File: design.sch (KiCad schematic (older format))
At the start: 20 parts, among them J1 USB_C_Receptacle, J2 Conn_01x05, Q1 2N7002K, Q2 2N7002K, Q3 2N7002K, U1 ATtiny814-SS

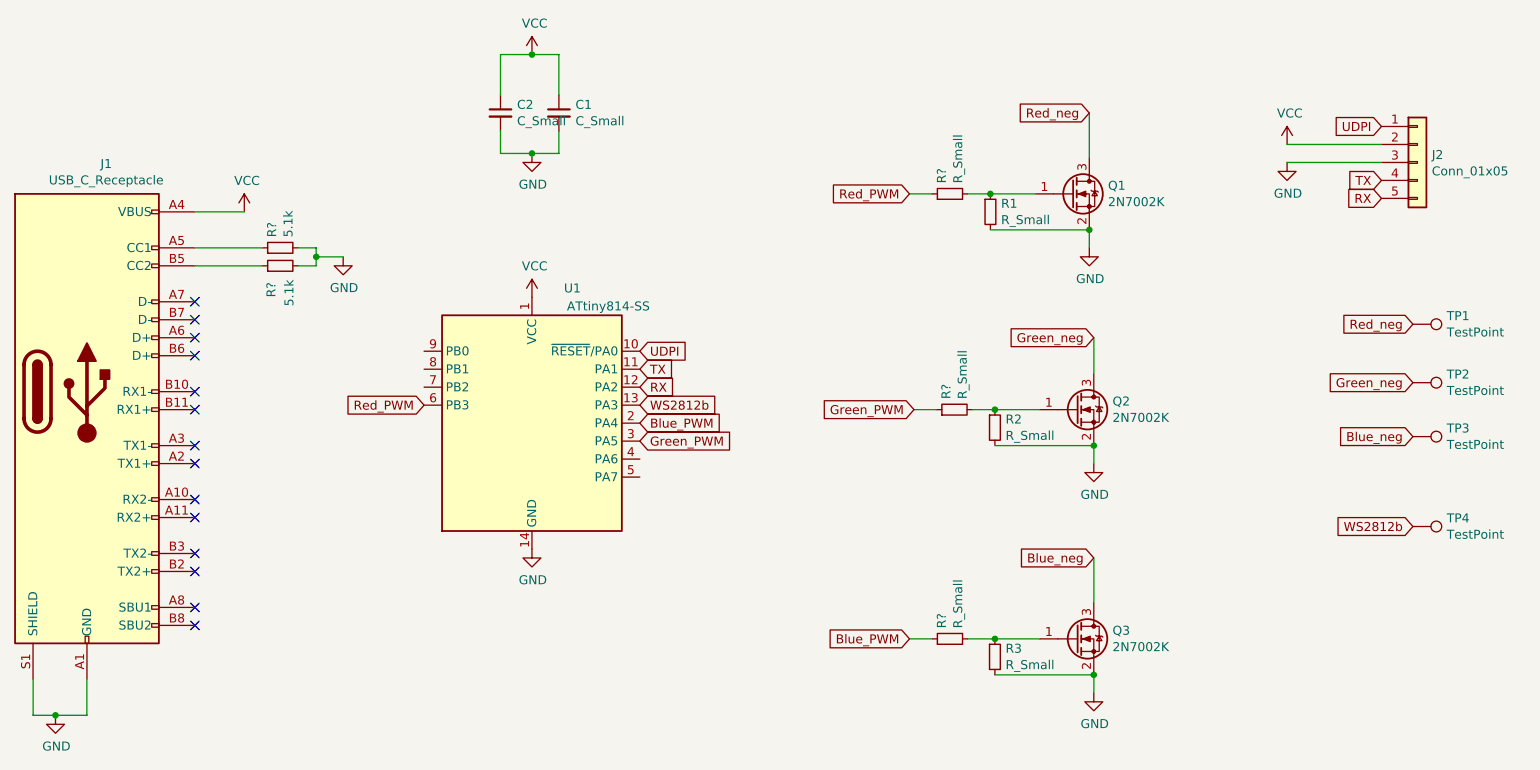
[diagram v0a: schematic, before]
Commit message: simple usb c footprint
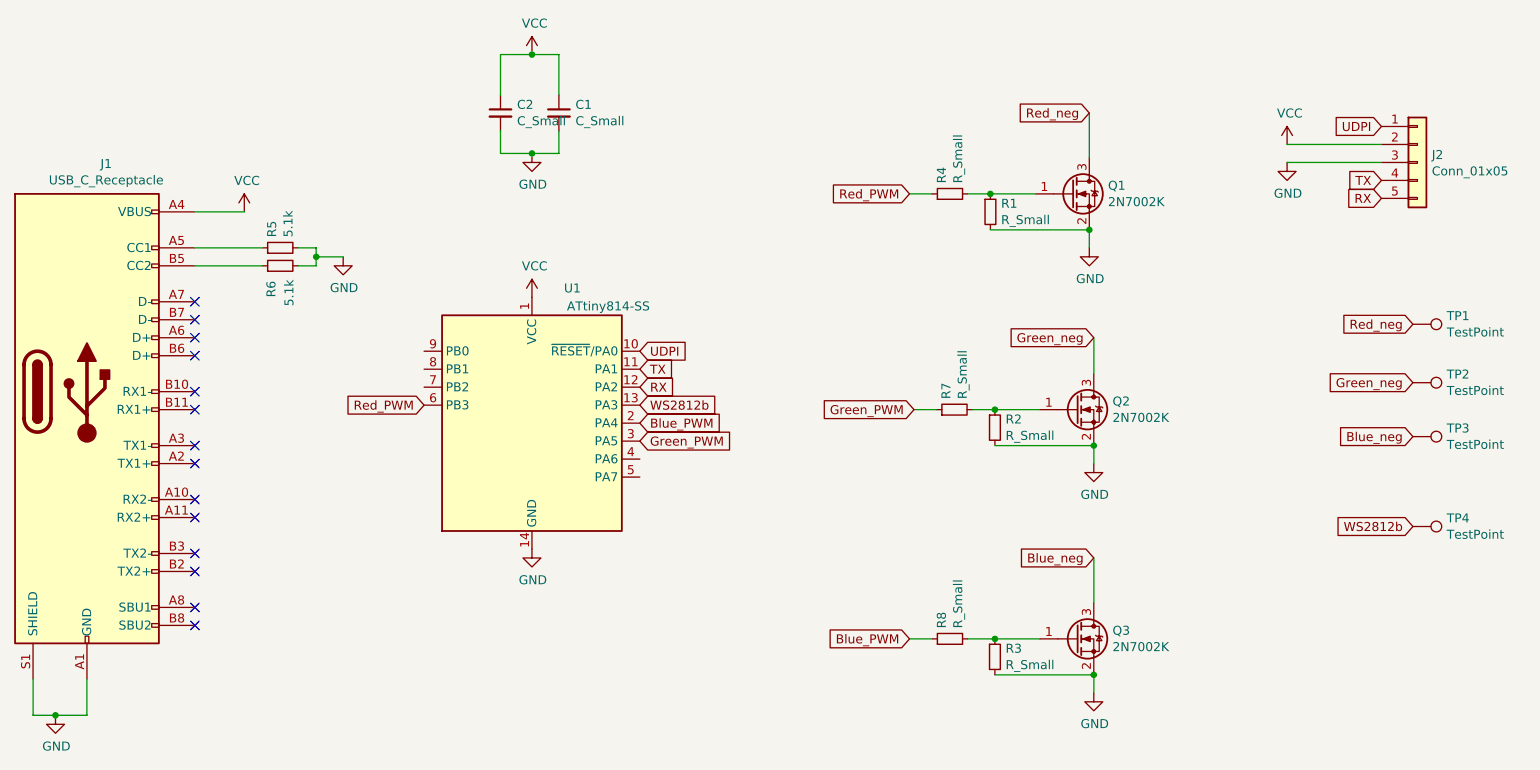
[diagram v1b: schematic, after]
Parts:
- J1: footprint Connector_USB:USB_C_Receptacle_HRO_TYPE-C-31-M-12 -> Connector_USB:USB_C_Receptacle_HRO_TYPE-C-31-M-12_simple
- J2: footprint E32-xxxT20D:UDPI_interface -> E32-xxxT20D:UDPI_interface_small
- gave numbers to parts that had none: 5
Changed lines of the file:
@@
 F 0 "J1" H 2207 4842 50  0000 C CNN
 F 1 "USB_C_Receptacle" H 2207 4751 50  0000 C CNN
-F 2 "Connector_USB:USB_C_Receptacle_HRO_TYPE-C-31-M-12" H 2250 3575 50  0001 C CNN
+F 2 "Connector_USB:USB_C_Receptacle_HRO_TYPE-C-31-M-12_simple" H 2250 3575 50  0001 C CNN
 F 3 "https://www.usb.org/sites/default/files/documents/usb_type-c.zip" H 2250 3575 50  0001 C CNN
 	1    2100 3575
@@
 F 0 "J2" H 9580 2342 50  0000 L CNN
 F 1 "Conn_01x05" H 9580 2251 50  0000 L CNN
-F 2 "E32-xxxT20D:UDPI_interface" H 9500 2300 50  0001 C CNN
+F 2 "E32-xxxT20D:UDPI_interface_small" H 9500 2300 50  0001 C CNN
 F 3 "~" H 9500 2300 50  0001 C CNN
 	1    9500 2300
@@
 Connection ~ 4575 1700
 $Comp
-L Device:R_Small R?
+L Device:R_Small R4
 U 1 1 61A6A719
 P 6900 2475
-F 0 "R?" H 6959 2521 50  0000 L CNN
+F 0 "R4" H 6959 2521 50  0000 L CNN
 F 1 "R_Small" H 6959 2430 50  0000 L CNN
 F 2 "Resistor_SMD:R_0805_2012Metric" H 6900 2475 50  0001 C CNN
@@
 	6675 2475 6800 2475
 $Comp
-L Device:R_Small R?
+L Device:R_Small R7
 U 1 1 61A6CC22
 P 6925 3675
-F 0 "R?" H 6984 3721 50  0000 L CNN
+F 0 "R7" H 6984 3721 50  0000 L CNN
 F 1 "R_Small" H 6984 3630 50  0000 L CNN
 F 2 "Resistor_SMD:R_0805_2012Metric" H 6925 3675 50  0001 C CNN
@@
 	6700 3675 6825 3675
 $Comp
-L Device:R_Small R?
+L Device:R_Small R8
 U 1 1 61A6D9D6
 P 6900 4950
-F 0 "R?" H 6959 4996 50  0000 L CNN
+F 0 "R8" H 6959 4996 50  0000 L CNN
 F 1 "R_Small" H 6959 4905 50  0000 L CNN
 F 2 "Resistor_SMD:R_0805_2012Metric" H 6900 4950 50  0001 C CNN
@@
 NoConn ~ 2700 4875
 $Comp
-L power:GND #PWR?
+L power:GND #PWR0110
 U 1 1 61A7334E
 P 1925 5375
-F 0 "#PWR?" H 1925 5125 50  0001 C CNN
+F 0 "#PWR0110" H 1925 5125 50  0001 C CNN
 F 1 "GND" H 1930 5202 50  0000 C CNN
 F 2 "" H 1925 5375 50  0001 C CNN
@@
 Connection ~ 1925 5375
 $Comp
-L power:VCC #PWR?
+L power:VCC #PWR0111
 U 1 1 61A74E6E
 P 2975 2575
-F 0 "#PWR?" H 2975 2425 50  0001 C CNN
+F 0 "#PWR0111" H 2975 2425 50  0001 C CNN
 F 1 "VCC" H 2990 2748 50  0000 C CNN
 F 2 "" H 2975 2575 50  0001 C CNN
@@
 	2975 2575 2700 2575
 $Comp
-L Device:R_Small R?
+L Device:R_Small R5
 U 1 1 61A75EA7
 P 3175 2775
-F 0 "R?" H 3234 2821 50  0000 L CNN
+F 0 "R5" H 3234 2821 50  0000 L CNN
 F 1 "5.1k" H 3234 2730 50  0000 L CNN
 F 2 "Resistor_SMD:R_0805_2012Metric" H 3175 2775 50  0001 C CNN
@@
 	2700 2875 3075 2875
 $Comp
-L Device:R_Small R?
+L Device:R_Small R6
 U 1 1 61A77F57
 P 3175 2875
-F 0 "R?" H 3000 2925 50  0000 L CNN
+F 0 "R6" H 3000 2925 50  0000 L CNN
 F 1 "5.1k" H 2950 2825 50  0000 L CNN
 F 2 "Resistor_SMD:R_0805_2012Metric" H 3175 2875 50  0001 C CNN
@@
 $EndComp
 $Comp
-L power:GND #PWR?
+L power:GND #PWR0112
 U 1 1 61A78369
 P 3525 2825
-F 0 "#PWR?" H 3525 2575 50  0001 C CNN
+F 0 "#PWR0112" H 3525 2575 50  0001 C CNN
 F 1 "GND" H 3530 2652 50  0000 C CNN
 F 2 "" H 3525 2825 50  0001 C CNN

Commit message: Revert "simple usb c footprint"
This reverts commit 12942baa332d339e718c995e44cede0abfa1d6b5.
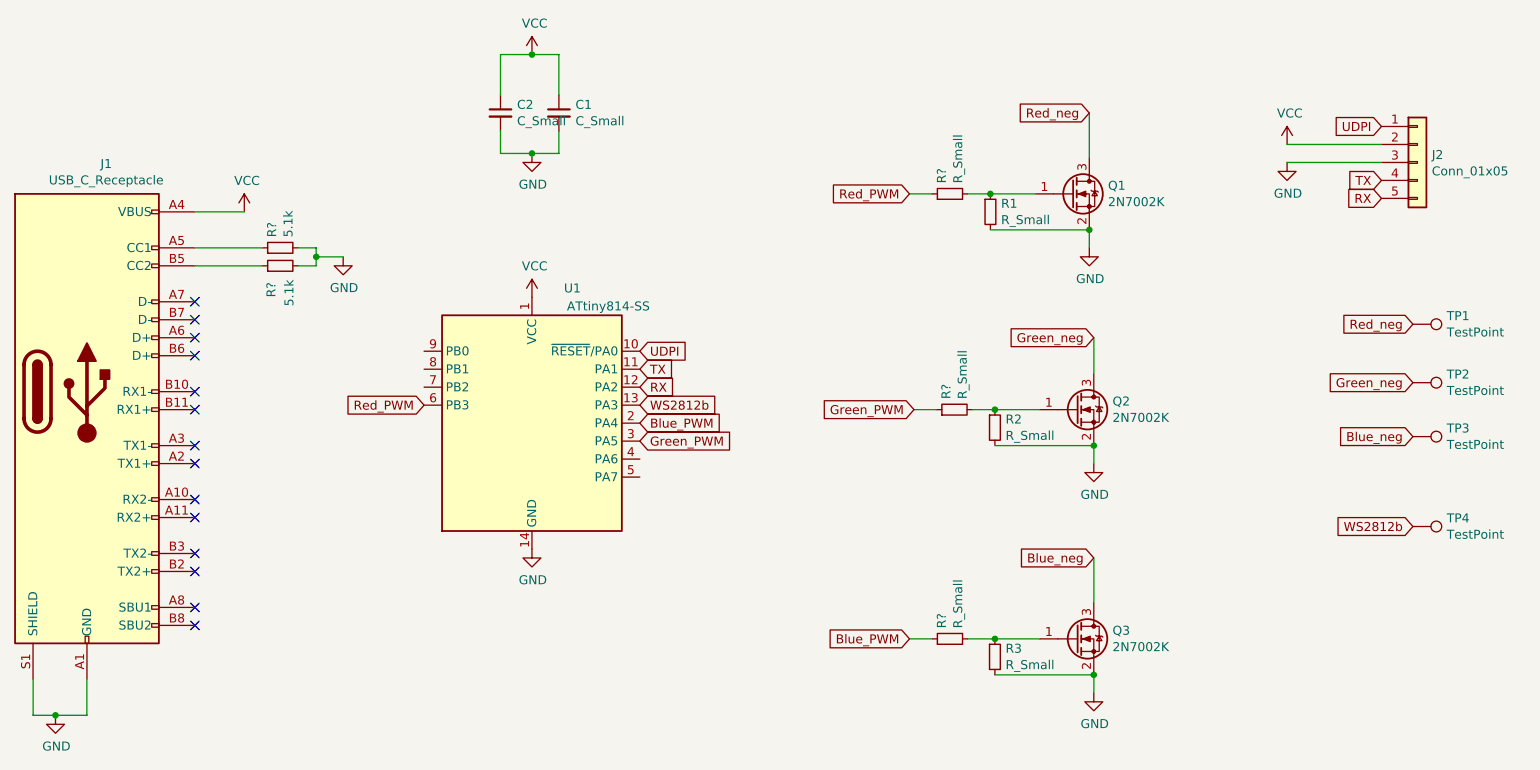
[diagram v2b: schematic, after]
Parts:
- J1: footprint Connector_USB:USB_C_Receptacle_HRO_TYPE-C-31-M-12_simple -> Connector_USB:USB_C_Receptacle_HRO_TYPE-C-31-M-12
- J2: footprint E32-xxxT20D:UDPI_interface_small -> E32-xxxT20D:UDPI_interface
- renumbered R4 to R?, R7 to R?, R8 to R?, R5 to R?, R6 to R?
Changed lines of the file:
@@
 F 0 "J1" H 2207 4842 50  0000 C CNN
 F 1 "USB_C_Receptacle" H 2207 4751 50  0000 C CNN
-F 2 "Connector_USB:USB_C_Receptacle_HRO_TYPE-C-31-M-12_simple" H 2250 3575 50  0001 C CNN
+F 2 "Connector_USB:USB_C_Receptacle_HRO_TYPE-C-31-M-12" H 2250 3575 50  0001 C CNN
 F 3 "https://www.usb.org/sites/default/files/documents/usb_type-c.zip" H 2250 3575 50  0001 C CNN
 	1    2100 3575
@@
 F 0 "J2" H 9580 2342 50  0000 L CNN
 F 1 "Conn_01x05" H 9580 2251 50  0000 L CNN
-F 2 "E32-xxxT20D:UDPI_interface_small" H 9500 2300 50  0001 C CNN
+F 2 "E32-xxxT20D:UDPI_interface" H 9500 2300 50  0001 C CNN
 F 3 "~" H 9500 2300 50  0001 C CNN
 	1    9500 2300
@@
 Connection ~ 4575 1700
 $Comp
-L Device:R_Small R4
+L Device:R_Small R?
 U 1 1 61A6A719
 P 6900 2475
-F 0 "R4" H 6959 2521 50  0000 L CNN
+F 0 "R?" H 6959 2521 50  0000 L CNN
 F 1 "R_Small" H 6959 2430 50  0000 L CNN
 F 2 "Resistor_SMD:R_0805_2012Metric" H 6900 2475 50  0001 C CNN
@@
 	6675 2475 6800 2475
 $Comp
-L Device:R_Small R7
+L Device:R_Small R?
 U 1 1 61A6CC22
 P 6925 3675
-F 0 "R7" H 6984 3721 50  0000 L CNN
+F 0 "R?" H 6984 3721 50  0000 L CNN
 F 1 "R_Small" H 6984 3630 50  0000 L CNN
 F 2 "Resistor_SMD:R_0805_2012Metric" H 6925 3675 50  0001 C CNN
@@
 	6700 3675 6825 3675
 $Comp
-L Device:R_Small R8
+L Device:R_Small R?
 U 1 1 61A6D9D6
 P 6900 4950
-F 0 "R8" H 6959 4996 50  0000 L CNN
+F 0 "R?" H 6959 4996 50  0000 L CNN
 F 1 "R_Small" H 6959 4905 50  0000 L CNN
 F 2 "Resistor_SMD:R_0805_2012Metric" H 6900 4950 50  0001 C CNN
@@
 NoConn ~ 2700 4875
 $Comp
-L power:GND #PWR0110
+L power:GND #PWR?
 U 1 1 61A7334E
 P 1925 5375
-F 0 "#PWR0110" H 1925 5125 50  0001 C CNN
+F 0 "#PWR?" H 1925 5125 50  0001 C CNN
 F 1 "GND" H 1930 5202 50  0000 C CNN
 F 2 "" H 1925 5375 50  0001 C CNN
@@
 Connection ~ 1925 5375
 $Comp
-L power:VCC #PWR0111
+L power:VCC #PWR?
 U 1 1 61A74E6E
 P 2975 2575
-F 0 "#PWR0111" H 2975 2425 50  0001 C CNN
+F 0 "#PWR?" H 2975 2425 50  0001 C CNN
 F 1 "VCC" H 2990 2748 50  0000 C CNN
 F 2 "" H 2975 2575 50  0001 C CNN
@@
 	2975 2575 2700 2575
 $Comp
-L Device:R_Small R5
+L Device:R_Small R?
 U 1 1 61A75EA7
 P 3175 2775
-F 0 "R5" H 3234 2821 50  0000 L CNN
+F 0 "R?" H 3234 2821 50  0000 L CNN
 F 1 "5.1k" H 3234 2730 50  0000 L CNN
 F 2 "Resistor_SMD:R_0805_2012Metric" H 3175 2775 50  0001 C CNN
@@
 	2700 2875 3075 2875
 $Comp
-L Device:R_Small R6
+L Device:R_Small R?
 U 1 1 61A77F57
 P 3175 2875
-F 0 "R6" H 3000 2925 50  0000 L CNN
+F 0 "R?" H 3000 2925 50  0000 L CNN
 F 1 "5.1k" H 2950 2825 50  0000 L CNN
 F 2 "Resistor_SMD:R_0805_2012Metric" H 3175 2875 50  0001 C CNN
@@
 $EndComp
 $Comp
-L power:GND #PWR0112
+L power:GND #PWR?
 U 1 1 61A78369
 P 3525 2825
-F 0 "#PWR0112" H 3525 2575 50  0001 C CNN
+F 0 "#PWR?" H 3525 2575 50  0001 C CNN
 F 1 "GND" H 3530 2652 50  0000 C CNN
 F 2 "" H 3525 2825 50  0001 C CNN
